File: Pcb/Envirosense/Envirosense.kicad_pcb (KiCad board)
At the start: 2 copper layers, 58.5 x 65 mm, 5 parts, among them J1 0.96" OLED, J2 Jack-DC, U2 L7805

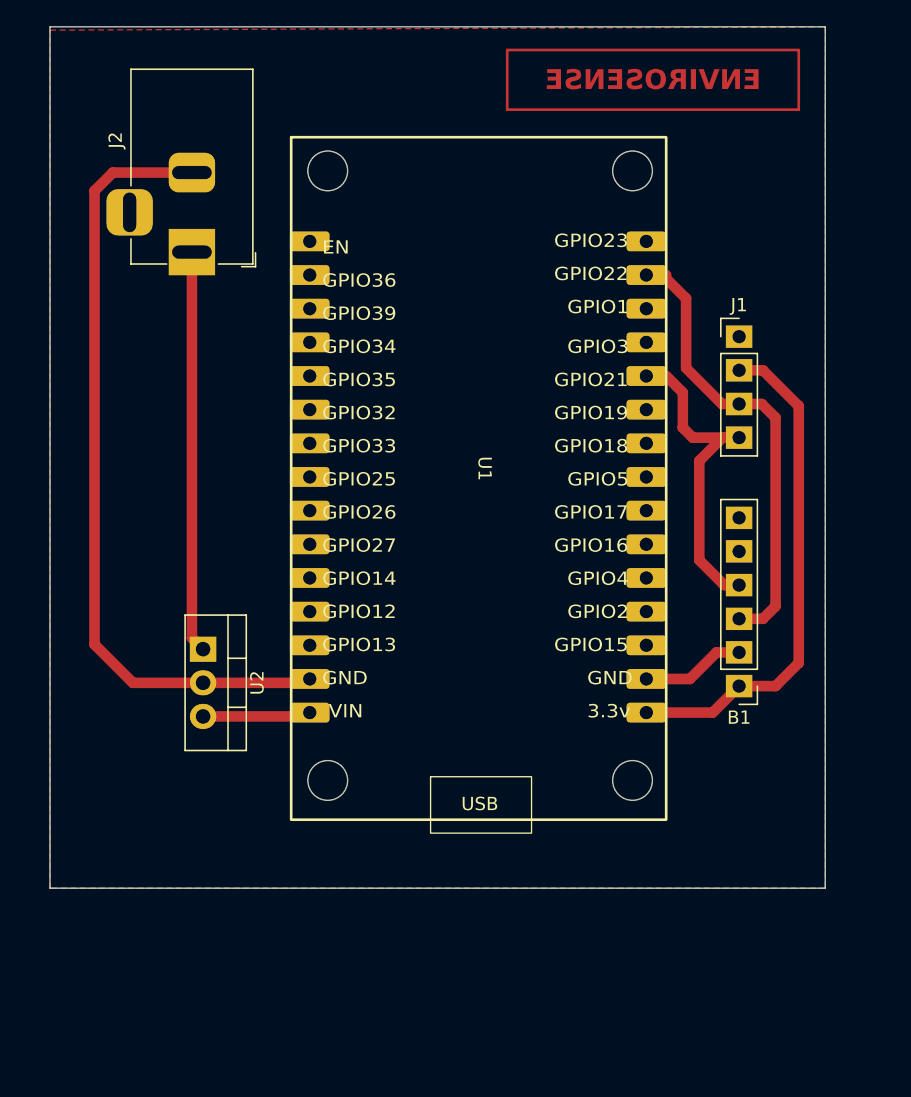
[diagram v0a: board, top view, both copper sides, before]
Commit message: Pcb
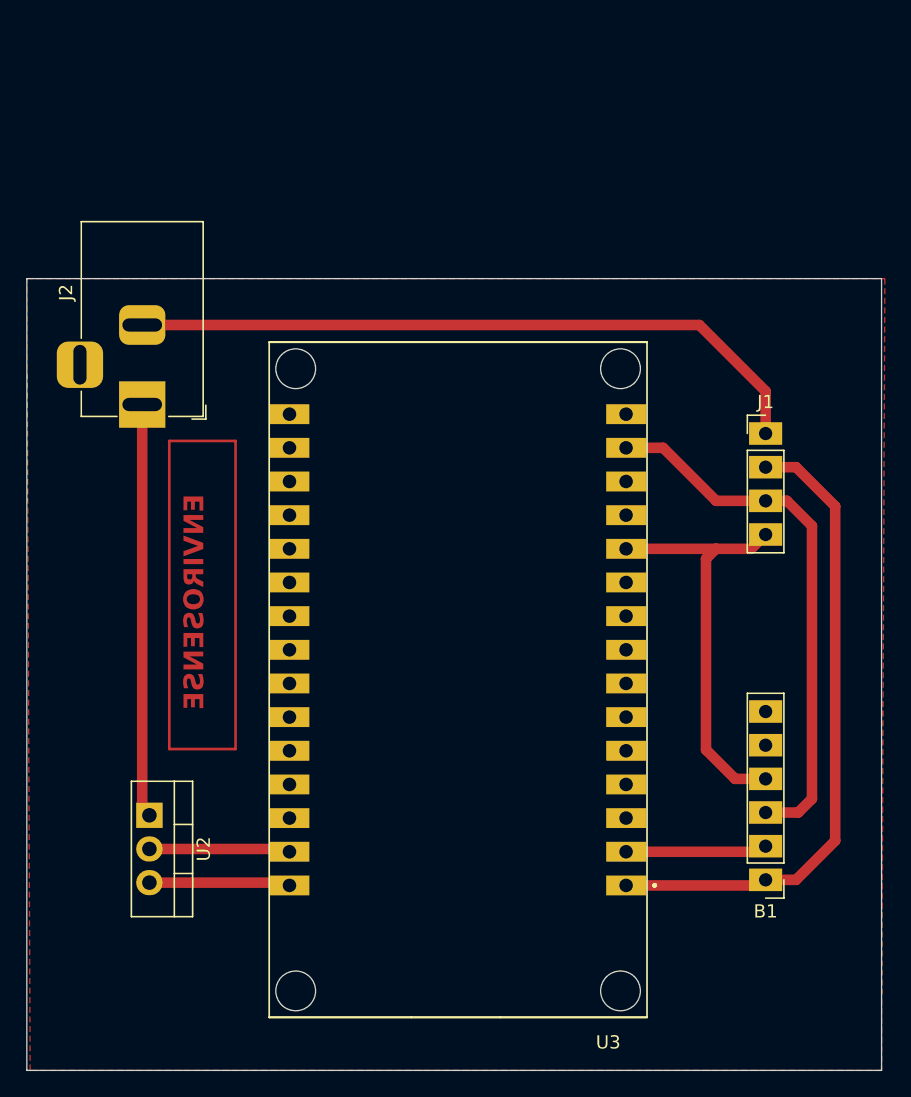
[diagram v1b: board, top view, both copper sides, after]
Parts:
- removed U1: ~, ESP32_Footprints:ESP32_30pin
- added U3: ESP32-DEVKIT-V1, ESP32-DEVKIT-V1:MODULE_ESP32_DEVKIT_V1, F.Cu at (138.8, 94.8)
- moved B1 14.8 mm to (162.0, 109.9)
- moved U2 13.2 mm to (115.5, 105.0)
- moved J2 12.1 mm to (115.0, 74.0)
- moved J1 7.58 mm to (162.0, 76.2)
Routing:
- net +3V3: track 38.1 -> 48.9 mm
- net SDA: track 25.5 -> 31.9 mm
- net GND: track 67.5 -> 73.7 mm
- net SCL: track 36.1 -> 41.0 mm
- net +5V: track 8.17 -> 10.7 mm
- net VCC: track 30.3 -> 31.2 mm
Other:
- board size 58.5 x 65 mm -> 64.5 x 59.8 mm
